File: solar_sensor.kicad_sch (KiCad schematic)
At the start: 3 parts

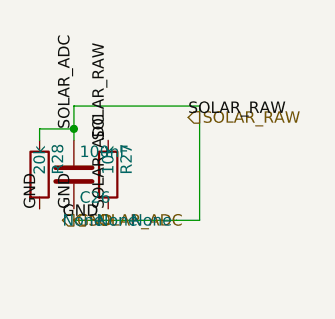
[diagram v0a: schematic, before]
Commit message: all unit test pass
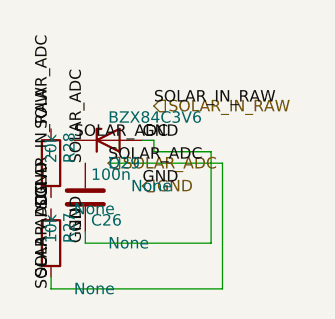
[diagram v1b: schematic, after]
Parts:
- added D29: BZX84C3V6, symbol Device:D_Zener
- C26: value 100nF -> 100n
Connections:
- net GND: now also D29.2 (A)
- net SOLAR_ADC: now also D29.1 (K)
- net SOLAR_RAW renamed SOLAR_IN_RAW
